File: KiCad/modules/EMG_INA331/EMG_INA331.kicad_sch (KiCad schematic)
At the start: 34 parts, among them J10 Conn_01x01_Pin, J13 Conn_01x01_Pin, J14 Conn_01x01_Pin, J15 Conn_01x01_Pin, J6 Conn_01x01_Pin, J7 Conn_01x01_Pin, J8 Conn_01x01_Pin, J9 Conn_01x01_Pin, U1 TLV9044IPWR, U2 AP2112K-3.3TRG1, U3 INA350ABSIDSGR_C4370677

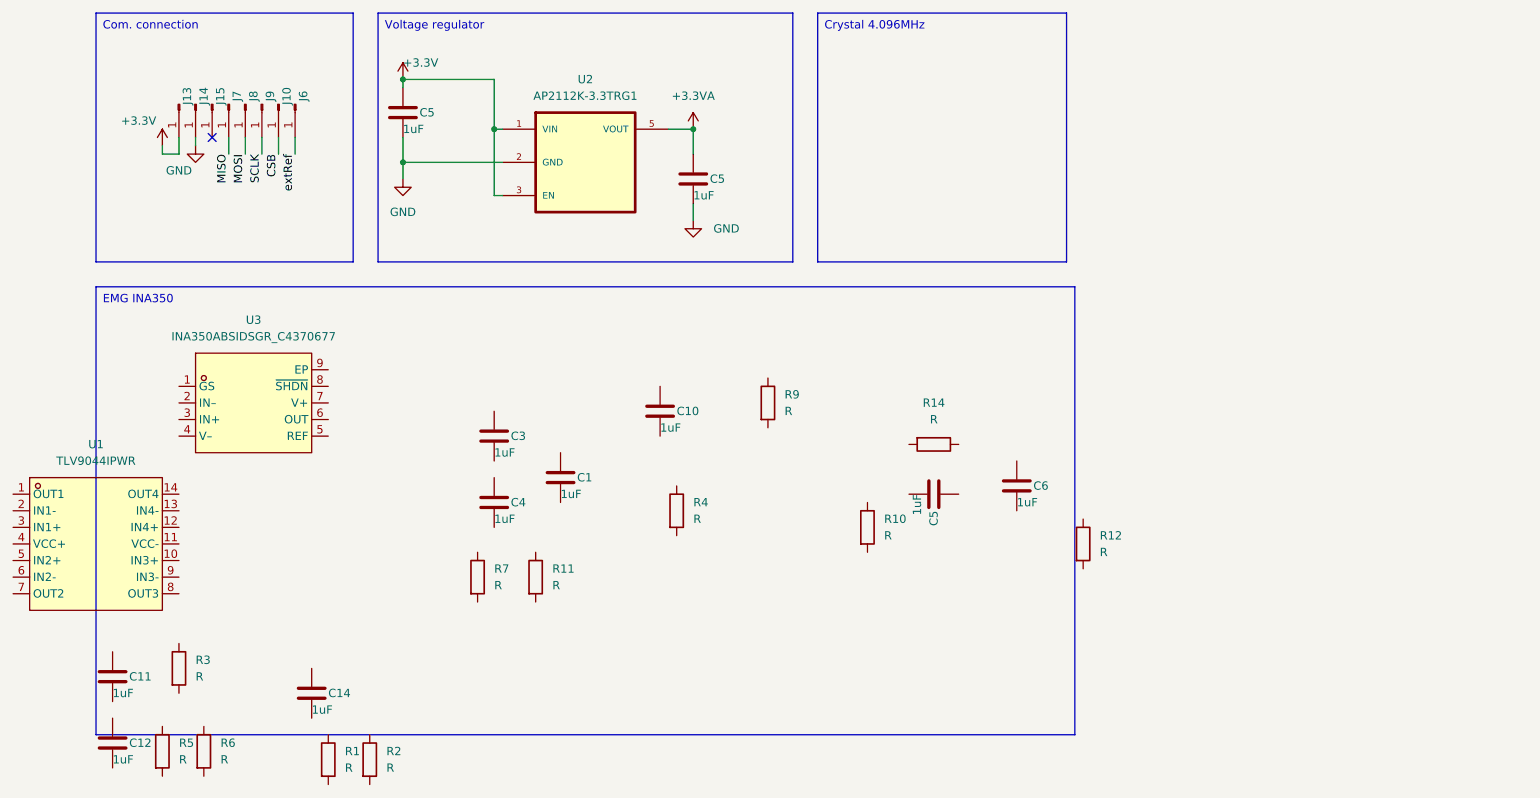
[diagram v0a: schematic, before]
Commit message: INA331 IMUICM
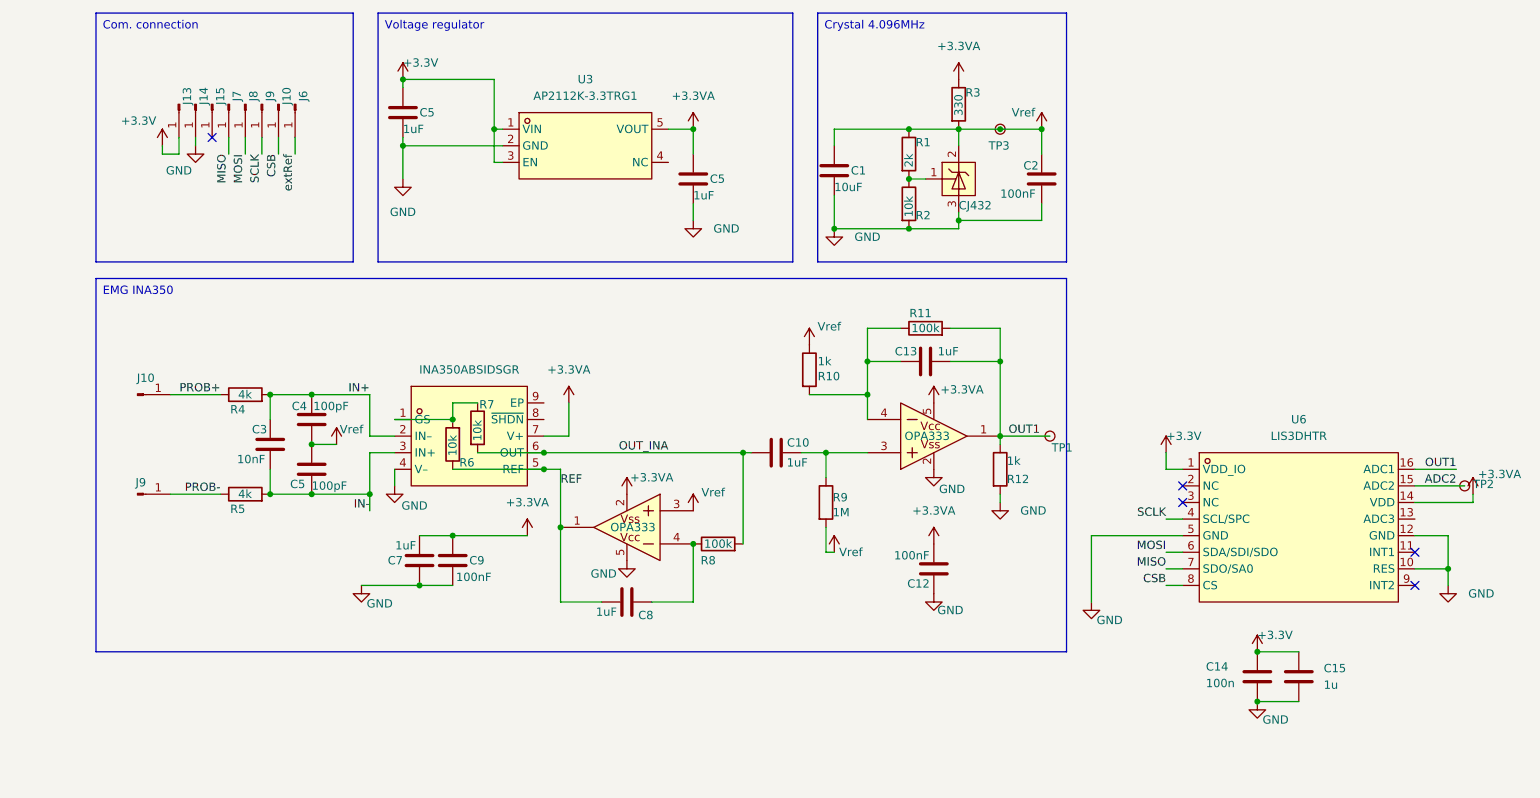
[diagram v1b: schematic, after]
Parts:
- removed C6: 1uF, Capacitor_SMD:C_0402_1005Metric, symbol Device:C
- removed R1, R10, R12, R14: R, Resistor_SMD:R_0201_0603Metric, symbol Device:R
- removed U1: TLV9044IPWR, 00_lcsc:TSSOP-14_L5.0-W4.4-P0.65-LS6.4-BL, symbol 00_lcsc:TLV9044IPWR
- removed U2: AP2112K-3.3TRG1, 00_custom-footprints:SOT95P285X140-5N, symbol 00_custom:AP2112K-3.3TRG1
- added C14: 100n, Capacitor_SMD:C_0402_1005Metric, symbol Device:C
- added C15: 1u, Capacitor_SMD:C_0402_1005Metric, symbol Device:C
- added C3: 10nF, Capacitor_SMD:C_0402_1005Metric, symbol Device:C
- added C7: 1uF, Capacitor_SMD:C_0402_1005Metric, symbol Device:C
- added C9: 100nF, Capacitor_SMD:C_0402_1005Metric, symbol Device:C
- added J10, J9: Conn_01x01_Pin, 00_custom-footprints:PinHeader_1x01_P1.27mm_Vertical, symbol Connector:Conn_01x01_Pin
- added R4, R5: 4k, Resistor_SMD:R_0402_1005Metric, symbol Device:R
- added R6, R7: 10k, Resistor_SMD:R_0402_1005Metric, symbol Device:R
- added TP1, TP2, TP3: TestPoint, 00_custom-footprints:TestPoint_Pad_D1.0mm, symbol 00_custom:TestPoint
- added U2, U4: OPA333, 00_lcsc:SOT-23-5_L2.9-W1.6-P0.95-LS2.8-BR, symbol 00_lcsc:OPA333M5_TR
- added U3: AP2112K-3.3TRG1, 00_lcsc:SOT-25-5_L2.9-W1.6-P0.95-LS2.8-BL, symbol 00_lcsc:AP2112K-3.3TRG1
- added U5: CJ432, 00_lcsc:SOT-23-3_L2.9-W1.3-P1.90-LS2.4-BR, symbol 00_lcsc:CJ432
- added U6: LIS3DHTR, 00_lcsc:LGA-16_L3.0-W3.0-P0.50-TL, symbol 00_lcsc:LIS3DHTR
- C1: renamed from C11; value 1uF -> 10uF
- C12: renamed from C1; value 1uF -> 100nF
- C2: renamed from C12; value 1uF -> 100nF
- C4, C5: value 1uF -> 100pF
- C5: footprint Capacitor_SMD:C_0201_0603Metric -> Capacitor_SMD:C_0402_1005Metric
- J10, J13, J14, J15, J6, J7, J8, J9: footprint Connector_PinHeader_1.27mm:PinHeader_1x01_P1.27mm_Vertical -> 00_custom-footprints:PinHeader_1x01_P1.27mm_Vertical
- R1: renamed from R5; value R -> 2k; footprint Resistor_SMD:R_0201_0603Metric -> Resistor_SMD:R_0402_1005Metric
- R10: renamed from R11; value R -> 1k; footprint Resistor_SMD:R_0201_0603Metric -> Resistor_SMD:R_0402_1005Metric
- R11: renamed from R9; value R -> 100k; footprint Resistor_SMD:R_0201_0603Metric -> Resistor_SMD:R_0402_1005Metric
- R12: renamed from R4; value R -> 1k; footprint Resistor_SMD:R_0201_0603Metric -> Resistor_SMD:R_0402_1005Metric
- R2: renamed from R3; value R -> 10k; footprint Resistor_SMD:R_0201_0603Metric -> Resistor_SMD:R_0402_1005Metric
- R3: renamed from R6; value R -> 330; footprint Resistor_SMD:R_0201_0603Metric -> Resistor_SMD:R_0402_1005Metric
- R8: renamed from R2; value R -> 100k; footprint Resistor_SMD:R_0201_0603Metric -> Resistor_SMD:R_0402_1005Metric
- R9: renamed from R7; value R -> 1M; footprint Resistor_SMD:R_0201_0603Metric -> Resistor_SMD:R_0402_1005Metric
- U1: renamed from U3; value INA350ABSIDSGR_C4370677 -> INA350ABSIDSGR
- renumbered C3 to C10, C10 to C13, C14 to C8
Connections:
- net +3.3V: now also C14.1, C15.1, U3.1 (VIN), U3.3 (EN), U6.1 (VDD_IO)
- net +3.3VA: now also C12.1, R3.1, U1.7 (V+), C7.2, C9.1, U2.2 (V-), U3.5 (VOUT), U4.5 (V+), U6.14 (VDD)
- net CSB: now also U6.8 (CS)
- net GND: now also C1.2, C12.2, C2.2, R12.2, R2.2, U1.4 (V–), C14.2, C15.2, C7.1, C9.2, U2.5 (V+), U3.2 (GND), U4.2 (V-), U5.3 (A), U6.10 (RES), U6.12 (GND), U6.5 (GND)
- net MISO: now also U6.7 (SDO/SA0)
- net MOSI: now also U6.6 (SDA/SDI/SDO)
- net SCLK: now also U6.4 (SCL/SPC)
- net Vref: now reaches C1.1
- net Vref: now also C2.1, C4.2, C5.1, R1.1, R10.1, R3.2, R9.2, TP3.1, U2.3 (+IN), U5.2 (K)
- net at R2.1: now also R1.2, U5.1 (R)
- net at R8.1: now also C8.2, U2.4 (-IN)
- net OUT_INA: now reaches R8.2
- net OUT_INA: now also C10.1, U1.6 (OUT), R7.2
- net at U1.1 (GS): now also R6.2, R7.1
- net IN+: now reaches U1.2 (IN–)
- net IN+: now also C4.1, C3.1, R4.2
- net IN-: now reaches U1.3 (IN+)
- net IN-: now also C5.2, C3.2, R5.2
- net REF: now reaches U1.5 (REF)
- net REF: now also C8.1, R6.1, U2.1 (OUT)
- net at R11.1: now also C13.1, R10.2, U4.4 (-IN)
- net OUT1: now reaches R11.2
- net OUT1: now also C13.2, R12.1, TP1.1, U4.1 (OUT), U6.16 (ADC1)
- net at C10.2: now also R9.1, U4.3 (+IN)
- new net ADC2: TP2.1, U6.15 (ADC2)
- new net PROB+: J10.1 (Pin_1), R4.1
- new net PROB-: J9.1 (Pin_1), R5.1
- no-connect marks 1 -> 5
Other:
- moved on the sheet: C1, C10, C12, C13, C2, C8, R1, R10, R11, R12, R2, R3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
